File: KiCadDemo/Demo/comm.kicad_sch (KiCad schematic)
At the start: 9 parts, among them J6 Comm, M2 BSS84, U5 MAX3486

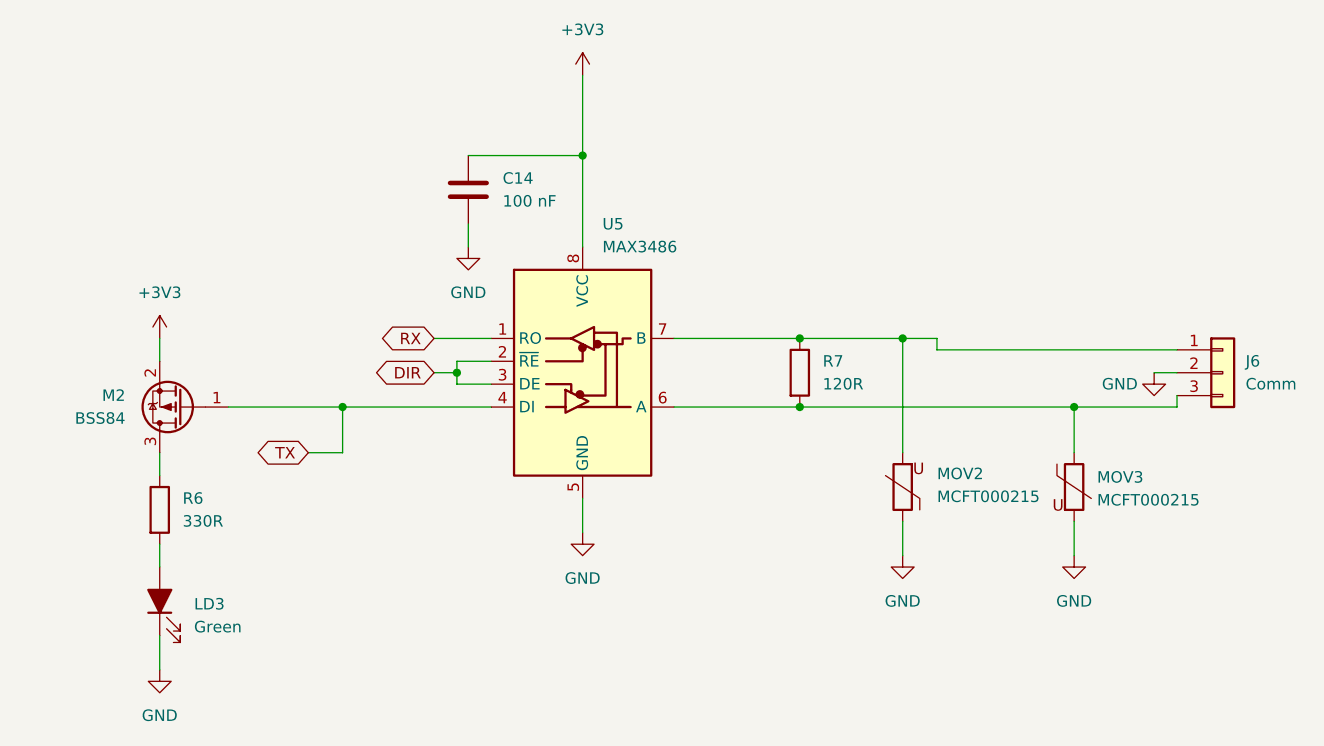
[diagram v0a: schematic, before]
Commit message: Add files via upload
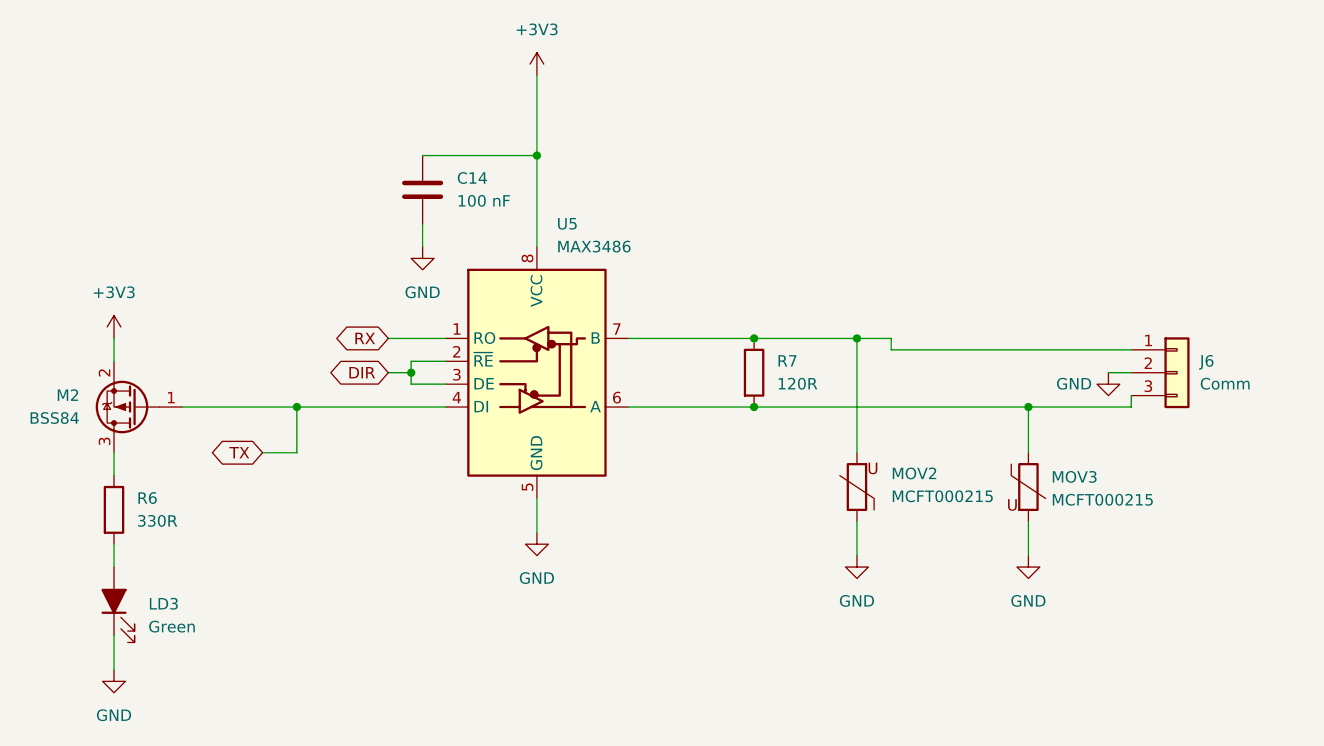
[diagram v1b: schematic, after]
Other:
- moved on the sheet: C14, J6, LD3, M2, MOV2, MOV3, R6, R7, U5

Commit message: Check #4
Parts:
- J6: footprint (none) -> Demo:IO3
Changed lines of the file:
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@@
       (effects (font (size 1.27 1.27)) (justify left))
     )
-    (property "Footprint" "" (at 208.28 86.36 0)
+    (property "Footprint" "Demo:IO3" (at 208.28 86.36 0)
       (effects (font (size 1.27 1.27)) hide)
     )
